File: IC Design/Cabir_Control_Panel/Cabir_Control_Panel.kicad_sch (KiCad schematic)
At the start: 20 parts

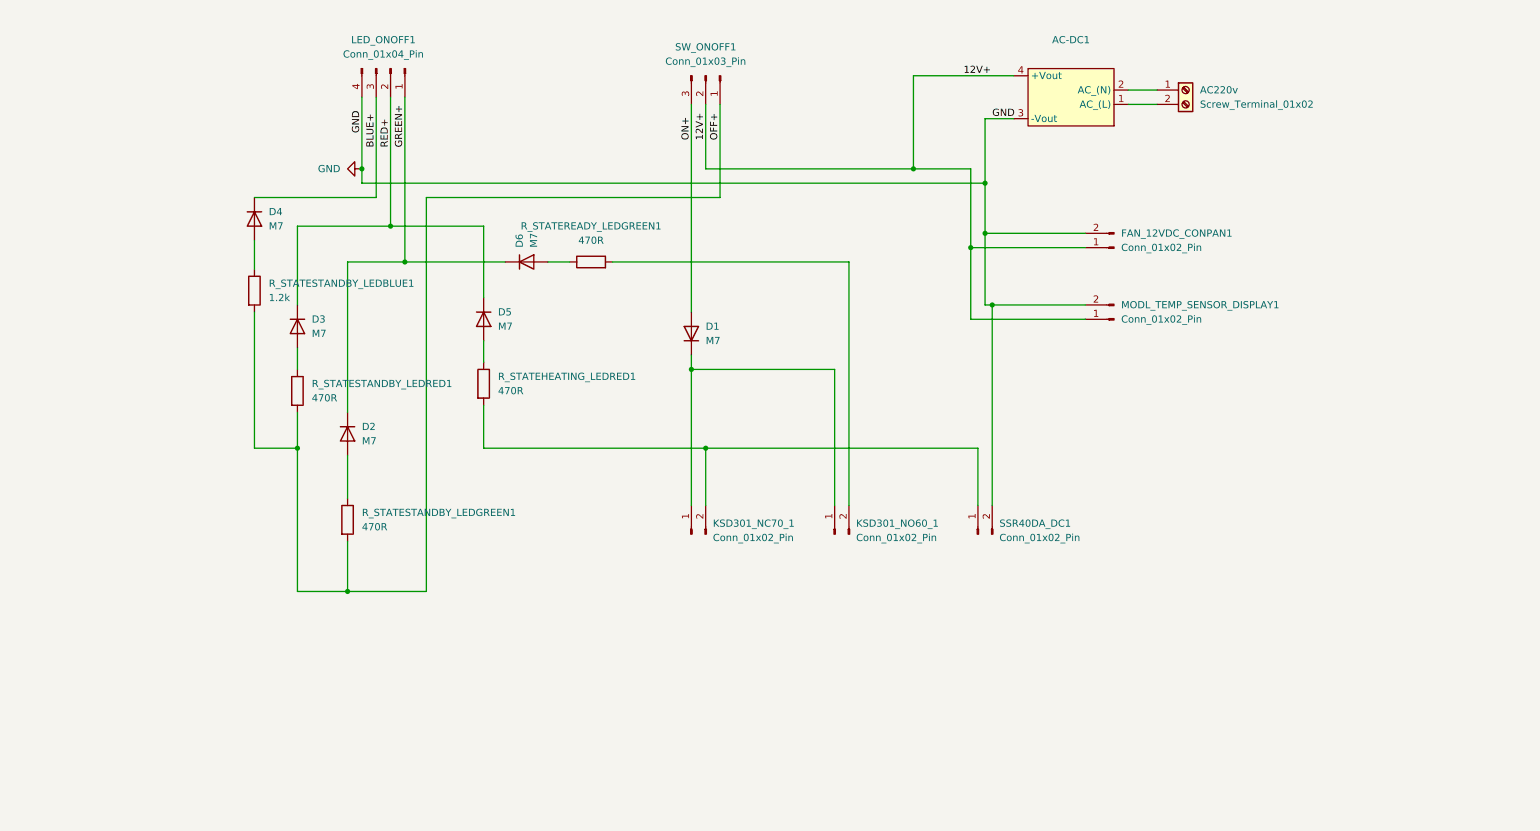
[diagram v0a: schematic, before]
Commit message: Circuit design - initial
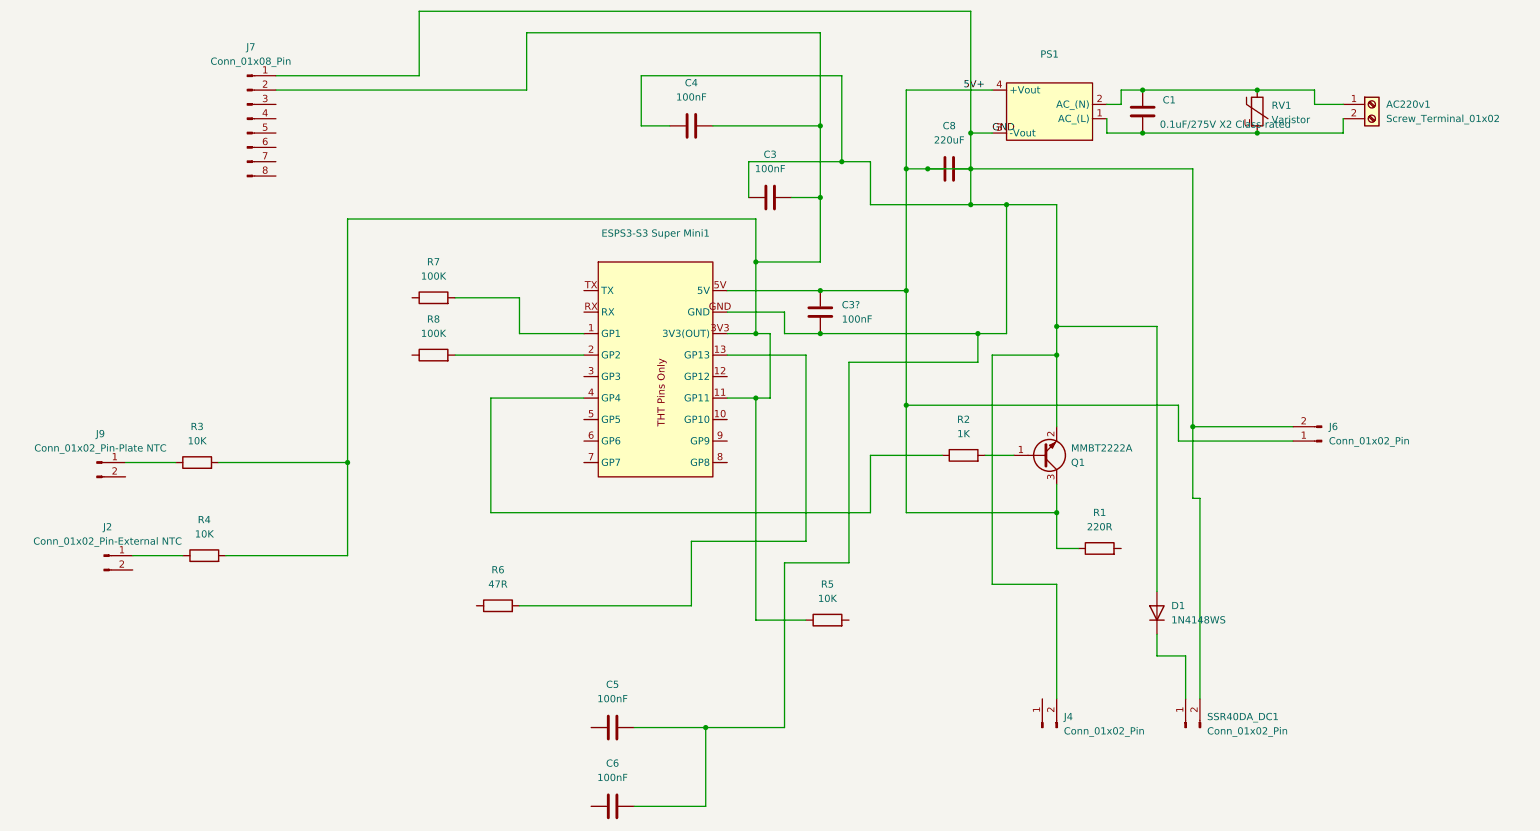
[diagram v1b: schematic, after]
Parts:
- removed D1, D2, D3, D4, D5, D6: M7, Diode_SMD:D_SMA_Handsoldering, symbol Device:D
- removed KSD301_NC70_1, MODL_TEMP_SENSOR_DISPLAY1: Conn_01x02_Pin, Connector_JST:JST_XH_B2B-XH-A_1x02_P2.50mm_Vertical, symbol Connector:Conn_01x02_Pin
- removed LED_ONOFF1: Conn_01x04_Pin, Connector_JST:JST_PH_B4B-PH-K_1x04_P2.00mm_Vertical, symbol Connector:Conn_01x04_Pin
- removed R_STATEHEATING_LEDRED1, R_STATEREADY_LEDGREEN1, R_STATESTANDBY_LEDGREEN1, R_STATESTANDBY_LEDRED1: 470R, Resistor_SMD:R_1206_3216Metric_Pad1.30x1.75mm_HandSolder, symbol Device:R
- removed R_STATESTANDBY_LEDBLUE1: 1.2k, Resistor_SMD:R_1206_3216Metric_Pad1.30x1.75mm_HandSolder, symbol Device:R
- removed SW_ONOFF1: Conn_01x03_Pin, Connector_JST:JST_PH_B3B-PH-K_1x03_P2.00mm_Vertical, symbol Connector:Conn_01x03_Pin
- added C1: 0.1uF/275V X2 Class-rated, symbol Device:C
- added C3, C3?, C4, C5, C6: 100nF, symbol Device:C
- added C8: 220uF, symbol Device:C
- added D1: 1N4148WS, Diode_SMD:D_SOD-323, symbol Diode:1N4148WS
- added ESPS3-S3 Super Mini1: ~, symbol TMB_Library:ESP32-S3_Super_Mini_THTONLY
- added J2: Conn_01x02_Pin-External NTC, Connector_JST:JST_PH_B2B-PH-K_1x02_P2.00mm_Vertical, symbol Connector:Conn_01x02_Pin
- added J7: Conn_01x08_Pin, Connector_JST:JST_XH_B8B-XH-A_1x08_P2.50mm_Vertical, symbol Connector:Conn_01x08_Pin
- added J9: Conn_01x02_Pin-Plate NTC, Connector_JST:JST_PH_B2B-PH-K_1x02_P2.00mm_Vertical, symbol Connector:Conn_01x02_Pin
- added Q1: MMBT2222A, Package_TO_SOT_SMD:SOT-23, symbol Transistor_BJT:MMBT2222A
- added R1: 220R, Resistor_SMD:R_1206_3216Metric_Pad1.30x1.75mm_HandSolder, symbol Device:R
- added R2: 1K, Resistor_SMD:R_1206_3216Metric_Pad1.30x1.75mm_HandSolder, symbol Device:R
- added R3, R4, R5: 10K, Resistor_SMD:R_1206_3216Metric_Pad1.30x1.75mm_HandSolder, symbol Device:R
- added R6: 47R, Resistor_SMD:R_1206_3216Metric_Pad1.30x1.75mm_HandSolder, symbol Device:R
- added R7, R8: 100K, Resistor_SMD:R_1206_3216Metric_Pad1.30x1.75mm_HandSolder, symbol Device:R
- added RV1: Varistor, Varistor:RV_Disc_D12mm_W5.8mm_P7.5mm, symbol Device:Varistor
- PS1: renamed from AC-DC1; footprint TMB_Library:HLK-5M12_PCB_AC-DC_Adapter -> TMB_Library:HLK-10M05_PCB_AC-DC_Adapter
- renumbered AC220v to AC220v1, KSD301_NO60_1 to J4, FAN_12VDC_CONPAN1 to J6
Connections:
- net 12V+ is gone; now on net 5V+: J6.1 (Pin_1), PS1.4 (+Vout)
- net GND is gone; now on net 5V+: J6.2 (Pin_2), PS1.3 (-Vout), SSR40DA_DC1.2 (Pin_2)
- net at AC220v1.2 (Pin_2), PS1.1 (AC_(L)): now also C1.2, RV1.2
- net at AC220v1.1 (Pin_1), PS1.2 (AC_(N)): now also C1.1, RV1.1
- net 5V+: now reaches J4.2 (Pin_2)
- net 5V+: now also C3.1, C3?.1, C3?.2, C4.1, C5.2, C6.2, C8.1, C8.2, D1.2 (A), ESPS3-S3 Super Mini1.5V, ESPS3-S3 Super Mini1.GND, J7.1 (Pin_1), Q1.2 (E), Q1.3 (C), R1.1
- net at SSR40DA_DC1.1 (Pin_1): now also D1.1 (K)
- new net: ESPS3-S3 Super Mini1.1 (GP1), R7.2
- new net: C3.2, C4.2, ESPS3-S3 Super Mini1.11 (GP11), ESPS3-S3 Super Mini1.3V3 (3V3(OUT)), J7.2 (Pin_2), R3.2, R4.2, R5.1
- new net: ESPS3-S3 Super Mini1.13 (GP13), R6.2
- new net: ESPS3-S3 Super Mini1.2 (GP2), R8.2
- new net: ESPS3-S3 Super Mini1.4 (GP4), R2.1
- new net: Q1.1 (B), R2.2
- new net: J2.1 (Pin_1), R4.1
- new net: J9.1 (Pin_1), R3.1
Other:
- moved on the sheet: AC220v1, J4, J6, PS1, SSR40DA_DC1
